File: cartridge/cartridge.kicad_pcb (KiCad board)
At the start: 2 copper layers, 31 parts, among them J1 J1B1211CCD, SW1 DS01-254-S-02BE, SW2 CL-SB-13B-01T‎, U1 Teensy4.1, U2 SN74CBTLV3126PWR, U3 SST39VF6401B

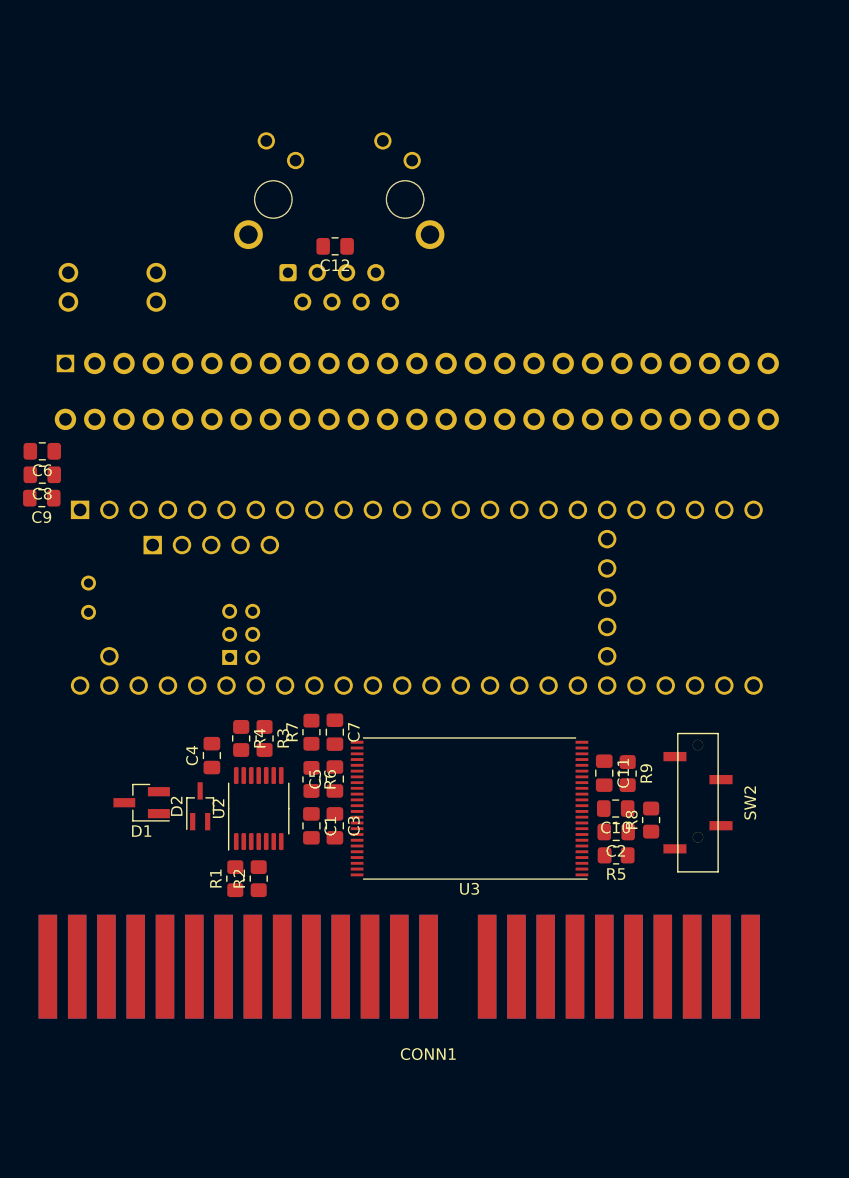
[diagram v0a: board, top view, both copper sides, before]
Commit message: WIP part layout
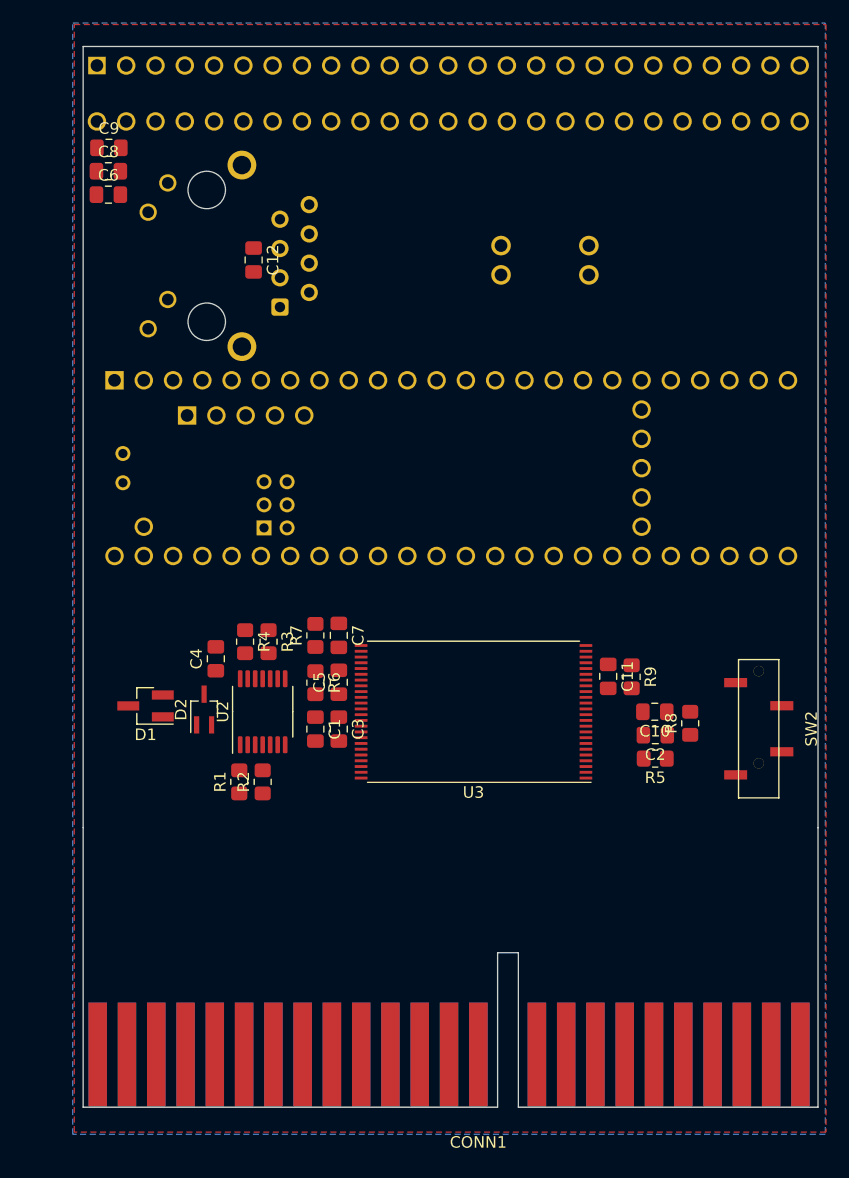
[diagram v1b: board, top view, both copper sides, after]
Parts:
- moved SW1 37.6 mm to (158.9, 68.3)
- moved C9 30.9 mm to (121.1, 58.5), turned to 0 degrees
- moved C8 26.9 mm to (121.1, 60.5), turned to 0 degrees
- moved CONN2 26.0 mm to (150.6, 53.9)
- moved C6 23.0 mm to (121.1, 62.6), turned to 0 degrees
- moved U1 11.6 mm to (150.8, 86.3)
- moved C10 9.05 mm to (168.5, 107.4)
- moved C2 9.05 mm to (168.5, 109.5)
- moved R8 9.05 mm to (171.5, 108.4)
- moved R5 9.05 mm to (168.5, 111.5)
- moved CONN1 8.76 mm to (122.7, 143.5)
- moved C1 8.40 mm to (139.0, 108.9)
- moved D1 8.40 mm to (124.3, 106.9)
- moved R2 8.40 mm to (134.5, 113.5)
- moved R4 8.40 mm to (132.9, 101.3)
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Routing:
- added copper zone on B.Cu, net GND
- added copper zone on F.Cu, net GND
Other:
- board outline added: 63.7 x 92 mm
- net class Default: clearance 0.2 -> 0.254
- net class Thin added: clearance 0.254, trace_width 0.127, via_dia 0.8, via_drill 0.4
- net class VCC added: clearance 0.3, trace_width 0.5, via_dia 0.8, via_drill 0.4
- rule trace_clearance: 0.2 -> 0.254
- rule trace_min: 0.2 -> 0.127
- rule via_min_size: 0.4 -> 0.6
